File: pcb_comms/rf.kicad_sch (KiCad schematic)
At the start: 25 parts, among them IC4 BGS12WN6E6329XTSA1, J6 SMA_CONNECTOR

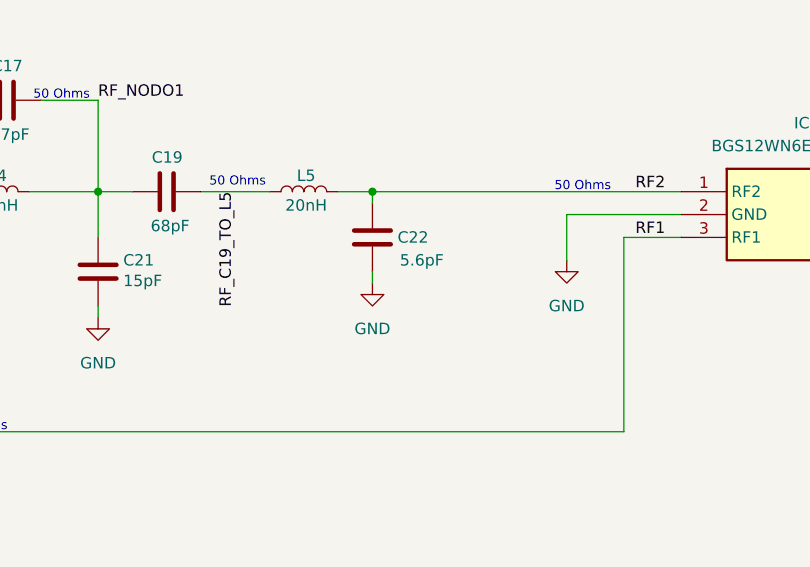
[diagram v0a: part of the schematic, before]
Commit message: PCB v2.1
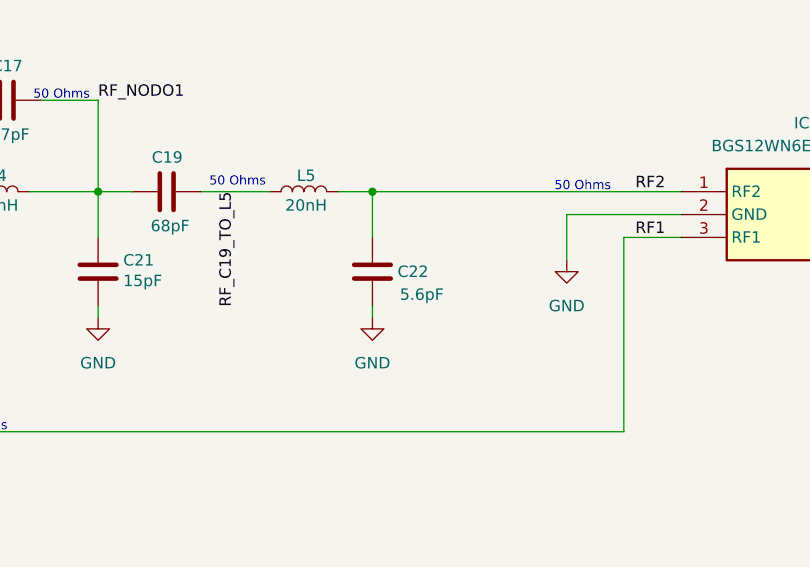
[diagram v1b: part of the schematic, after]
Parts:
- C17, C21, C22, C24, C28, C29: footprint Capacitor_SMD:C_0805_2012Metric_Pad1.18x1.45mm_HandSolder -> Capacitor_SMD:C_0603_1608Metric_Pad1.08x0.95mm_HandSolder
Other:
- moved on the sheet: C22

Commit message: Add STM32 gps test 1
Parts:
- L5: footprint Inductor_SMD:L_0402_1005Metric_Pad0.77x0.64mm_HandSolder -> Inductor_SMD:L_0603_1608Metric_Pad1.05x0.95mm_HandSolder
- L6: footprint Inductor_SMD:L_0402_1005Metric_Pad0.77x0.64mm_HandSolder -> Resistor_SMD:R_0603_1608Metric_Pad0.98x0.95mm_HandSolder
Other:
- company: Sanie Peralta, Alejandro Campo -> Sanie Peralta
- title: PC1: APRS & GPS -> PAYLOAD 1: APRS
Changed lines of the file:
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@@
 	(paper "A4")
 	(title_block
-		(title "PC1: APRS & GPS")
+		(title "PAYLOAD 1: APRS")
 		(date "2026-04-01")
-		(rev "1.0")
-		(company "Sanie Peralta, Alejandro Campo")
+		(rev "1.1")
+		(company "Sanie Peralta")
 		(comment 1 "Introducción a la Ingeniería Satelital ")
-		(comment 2 "Primer Parcial")
 	)
 	(text "50 Ohms"
@@
 			)
 		)
-		(property "Footprint" "Inductor_SMD:L_0402_1005Metric_Pad0.77x0.64mm_HandSolder"
+		(property "Footprint" "Inductor_SMD:L_0603_1608Metric_Pad1.05x0.95mm_HandSolder"
 			(at 119.38 52.07 0)
 			(effects
@@
 			)
 		)
-		(property "Footprint" "Inductor_SMD:L_0402_1005Metric_Pad0.77x0.64mm_HandSolder"
+		(property "Footprint" "Resistor_SMD:R_0603_1608Metric_Pad0.98x0.95mm_HandSolder"
 			(at 62.23 64.77 0)
 			(effects
